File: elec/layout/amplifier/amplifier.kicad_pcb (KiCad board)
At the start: 2 copper layers, 29 parts, among them U1 _Texas_Instruments_TAS5825MRH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

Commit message: builds working
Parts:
- C10, C6, C9: value (none) -> 680nF ±10% 50V X7R
- C14, C15: value (none) -> 22µF ±20% 25V X5R
- C16, C17, C18: value (none) -> 100nF ±10% 16V X7R
- C19, C2: value (none) -> 1µF ±10% 25V X5R
- C4, C7, C8: value (none) -> 470nF ±10% 50V X7R
- L2, L3, L4: value (none) -> 10µH ±20% 4.5A 68mΩ
- R3, R4, R5: value (none) -> 10kΩ ±1% 62.5mW
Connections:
- net DVDD renamed hv
- C1 pad 1: net-12 -> net-6
- C1 pad 2: net-2 -> net
- C10 pad 1: signal-3 -> signal-1
- C10 pad 2: net-2 -> net
- C11 pad 2: net-2 -> net
- C12 pad 2: net-2 -> net
- C13 pad 1: PVDD -> net-4
- C13 pad 2: net-2 -> net
- C14 pad 1: PVDD -> net-4
- C14 pad 2: net-2 -> net
- C15 pad 1: PVDD -> net-4
- C15 pad 2: net-2 -> net
- C16 pad 1: PVDD -> net-4
- C16 pad 2: net-2 -> net
- C17 pad 1: PVDD -> net-4
- C17 pad 2: net-2 -> net
- C18 pad 1: PVDD -> net-4
- C18 pad 2: net-2 -> net
- C19 pad 1: net-5 -> net-12
- C19 pad 2: net-2 -> net
- C2 pad 1: net-16 -> net-5
- C2 pad 2: net-2 -> net
- C3 pad 1: net-13 -> net-10
- C3 pad 2: net-14 -> net-8
- C4 pad 1: net-7 -> net-13
- C4 pad 2: net-8 -> net-14
- C5 pad 2: net-2 -> net
- C6 pad 1: signal-1 -> signal-2
- C6 pad 2: net-2 -> net
- C7 pad 1: net -> net-1
- C7 pad 2: net-1 -> net-2
- C8 pad 1: net-4 -> net-11
- C8 pad 2: net-3 -> net-7
- C9 pad 1: signal-2 -> signal-3
- C9 pad 2: net-2 -> net
- L1 pad 1: net-14 -> net-8
- L2 pad 1: net-8 -> net-14
- L2 pad 2: signal-1 -> signal-2
- L3 pad 1: net-1 -> net-2
- L3 pad 2: signal-2 -> signal-3
- L4 pad 1: net-3 -> net-7
- L4 pad 2: signal-3 -> signal-1
- R1 pad 1: net-10 -> net-3
- R1 pad 2: net-2 -> net
- R2 pad 1: net-6 -> net-15
- R3 pad 1: net-11 -> net-16
- R4 pad 1: net-9 -> net-17
- R5 pad 1: net-15 -> net-9
- U1 pad 1: net-7 -> net-13
- U1 pad 10: net-11 -> net-16
- U1 pad 11: net-15 -> net-9
- U1 pad 17: net-9 -> net-17
- U1 pad 18: net-16 -> net-5
- U1 pad 19: net-12 -> net-6
- U1 pad 2: net-8 -> net-14
- U1 pad 20: net-2 -> net
- U1 pad 21: PVDD -> net-4
- U1 pad 22: PVDD -> net-4
- U1 pad 23: net-3 -> net-7
- U1 pad 24: net-4 -> net-11
- U1 pad 25: net-2 -> net
- U1 pad 26: net-2 -> net
- U1 pad 27: net-1 -> net-2
- U1 pad 28: net -> net-1
- U1 pad 29: net-13 -> net-10
- U1 pad 3: PVDD -> net-4
- U1 pad 30: net-14 -> net-8
- U1 pad 31: net-2 -> net
- U1 pad 32: net-2 -> net
- U1 pad 33: net-2 -> net
- U1 pad 4: PVDD -> net-4
- U1 pad 5: net-2 -> net
- U1 pad 7: net-5 -> net-12
- U1 pad 8: net-10 -> net-3
- U1 pad 9: net-6 -> net-15
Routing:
- net (no net): track 50.8 -> 65.3 mm
- net PVDD: track 14.5 -> 0.00 mm
- removed copper zone on F.Cu, net PVDD

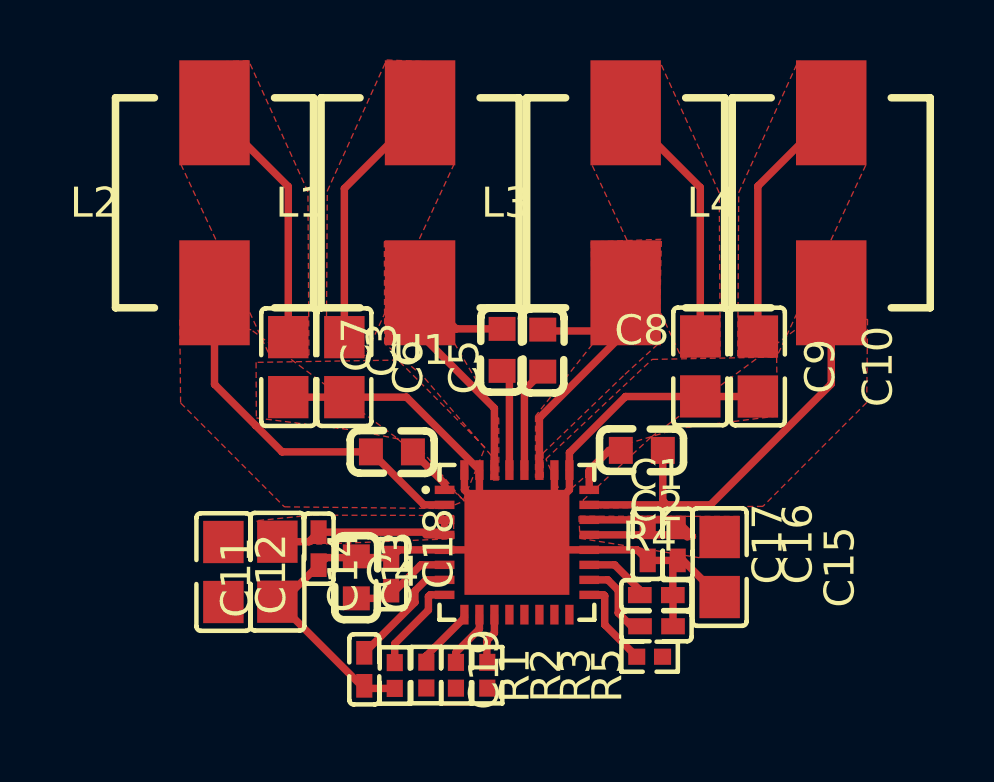
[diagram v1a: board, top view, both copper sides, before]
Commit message: Build full
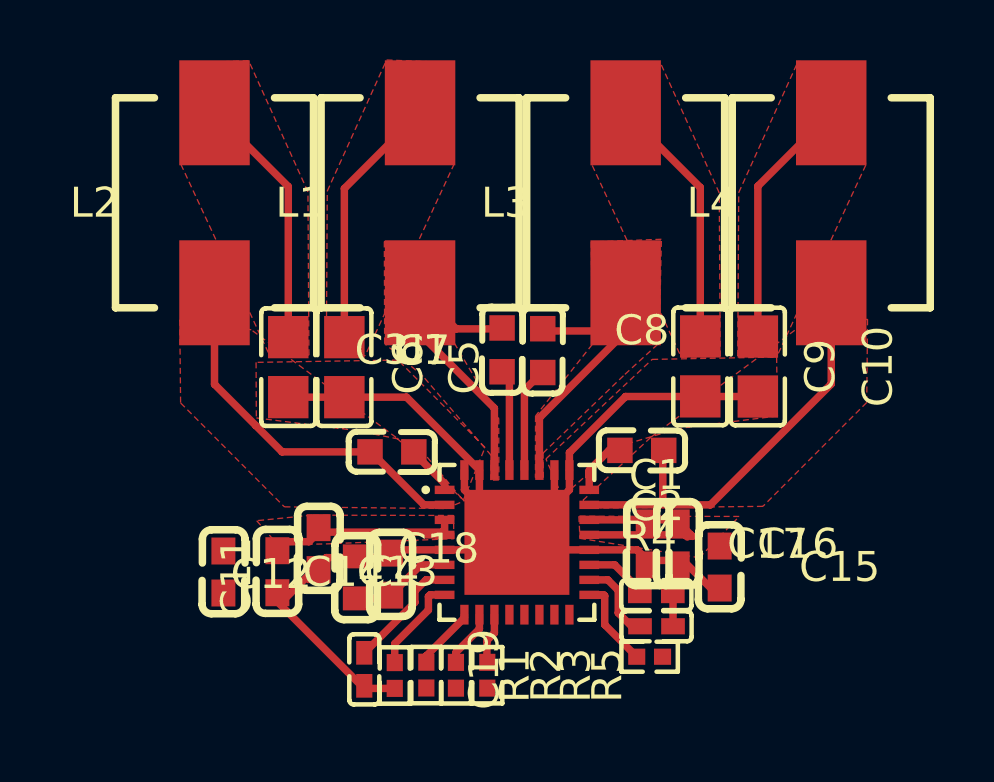
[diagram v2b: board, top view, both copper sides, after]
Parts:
- C1, C19, C2: value 1µF ±10% 25V X5R -> 1µF ±10% 10V X5R
- C11: value 4.7µF ±10% 16V X5R -> 100nF ±10% 50V X7R
- C12, C16, C17, C18: value 100nF ±10% 16V X7R -> 100nF ±10% 50V X7R; footprint lcsc:C0402 -> lcsc:C0603
- C13, C14, C15: value 22µF ±20% 25V X5R -> 100nF ±10% 50V X7R; footprint lcsc:C0805 -> lcsc:C0603
- C3, C4, C7, C8: footprint lcsc:C0603 -> lcsc:CAP-SMD_L1.6-W0.8-3
- L1, L2, L3, L4: value 10µH ±20% 4.5A 68mΩ -> 10µH ±20% infHz 4.5A 68mΩ
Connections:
- net fault-hv renamed hv-3
- net mute-hv renamed hv-1
- net pdn-hv renamed hv-4
- C1 pad 1: net-6 -> net-10
- C1 pad 2: net -> net-4
- C10 pad 1: signal-1 -> signal-2
- C10 pad 2: net -> net-4
- C11 pad 1: hv -> hv-2
- C11 pad 2: net -> net-4
- C12 pad 1: hv -> hv-2
- C12 pad 2: net -> net-4
- C13 pad 1: net-4 -> net-5
- C13 pad 2: net -> net-4
- C14 pad 1: net-4 -> net-5
- C14 pad 2: net -> net-4
- C15 pad 1: net-4 -> net-5
- C15 pad 2: net -> net-4
- C16 pad 1: net-4 -> net-5
- C16 pad 2: net -> net-4
- C17 pad 1: net-4 -> net-5
- C17 pad 2: net -> net-4
- C18 pad 1: net-4 -> net-5
- C18 pad 2: net -> net-4
- C19 pad 1: net-12 -> net-11
- C19 pad 2: net -> net-4
- C2 pad 1: net-5 -> net-3
- C2 pad 2: net -> net-4
- C3 pad 1: net-10 -> net-14
- C3 pad 2: net-8 -> net-9
- C4 pad 1: net-13 -> net-7
- C4 pad 2: net-14 -> net-8
- C5 pad 1: signal -> signal-1
- C5 pad 2: net -> net-4
- C6 pad 1: signal-2 -> signal-3
- C6 pad 2: net -> net-4
- C7 pad 1: net-1 -> net
- C7 pad 2: net-2 -> net-1
- C8 pad 1: net-11 -> net-16
- C8 pad 2: net-7 -> net-13
- C9 pad 1: signal-3 -> signal
- C9 pad 2: net -> net-4
- L1 pad 1: net-8 -> net-9
- L1 pad 2: signal -> signal-1
- L2 pad 1: net-14 -> net-8
- L2 pad 2: signal-2 -> signal-3
- L3 pad 1: net-2 -> net-1
- L3 pad 2: signal-3 -> signal
- L4 pad 1: net-7 -> net-13
- L4 pad 2: signal-1 -> signal-2
- R1 pad 1: net-3 -> net-12
- R1 pad 2: net -> net-4
- R2 pad 1: net-15 -> net-17
- R3 pad 1: net-16 -> net-6
- R4 pad 1: net-17 -> net-15
- R5 pad 1: net-9 -> net-2
- R5 pad 2: warn-hv -> hv
- U1 pad 1: net-13 -> net-7
- U1 pad 10: net-16 -> net-6
- U1 pad 11: net-9 -> net-2
- U1 pad 17: net-17 -> net-15
- U1 pad 18: net-5 -> net-3
- U1 pad 19: net-6 -> net-10
- U1 pad 2: net-14 -> net-8
- U1 pad 20: net -> net-4
- U1 pad 21: net-4 -> net-5
- U1 pad 22: net-4 -> net-5
- U1 pad 23: net-7 -> net-13
- U1 pad 24: net-11 -> net-16
- U1 pad 25: net -> net-4
- U1 pad 26: net -> net-4
- U1 pad 27: net-2 -> net-1
- U1 pad 28: net-1 -> net
- U1 pad 29: net-10 -> net-14
- U1 pad 3: net-4 -> net-5
- U1 pad 30: net-8 -> net-9
- U1 pad 31: net -> net-4
- U1 pad 32: net -> net-4
- U1 pad 33: net -> net-4
- U1 pad 4: net-4 -> net-5
- U1 pad 5: net -> net-4
- U1 pad 6: hv -> hv-2
- U1 pad 7: net-12 -> net-11
- U1 pad 8: net-3 -> net-12
- U1 pad 9: net-15 -> net-17
